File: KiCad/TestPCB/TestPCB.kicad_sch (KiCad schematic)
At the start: 42 parts, among them J1 USB_C_Receptacle_PowerOnly_6P, Q5 2N7000, Q6 2N7000, U1 ESP32-S3-WROOM-1, U1 MCP73831-2-OT, U2 TC1185-xCT

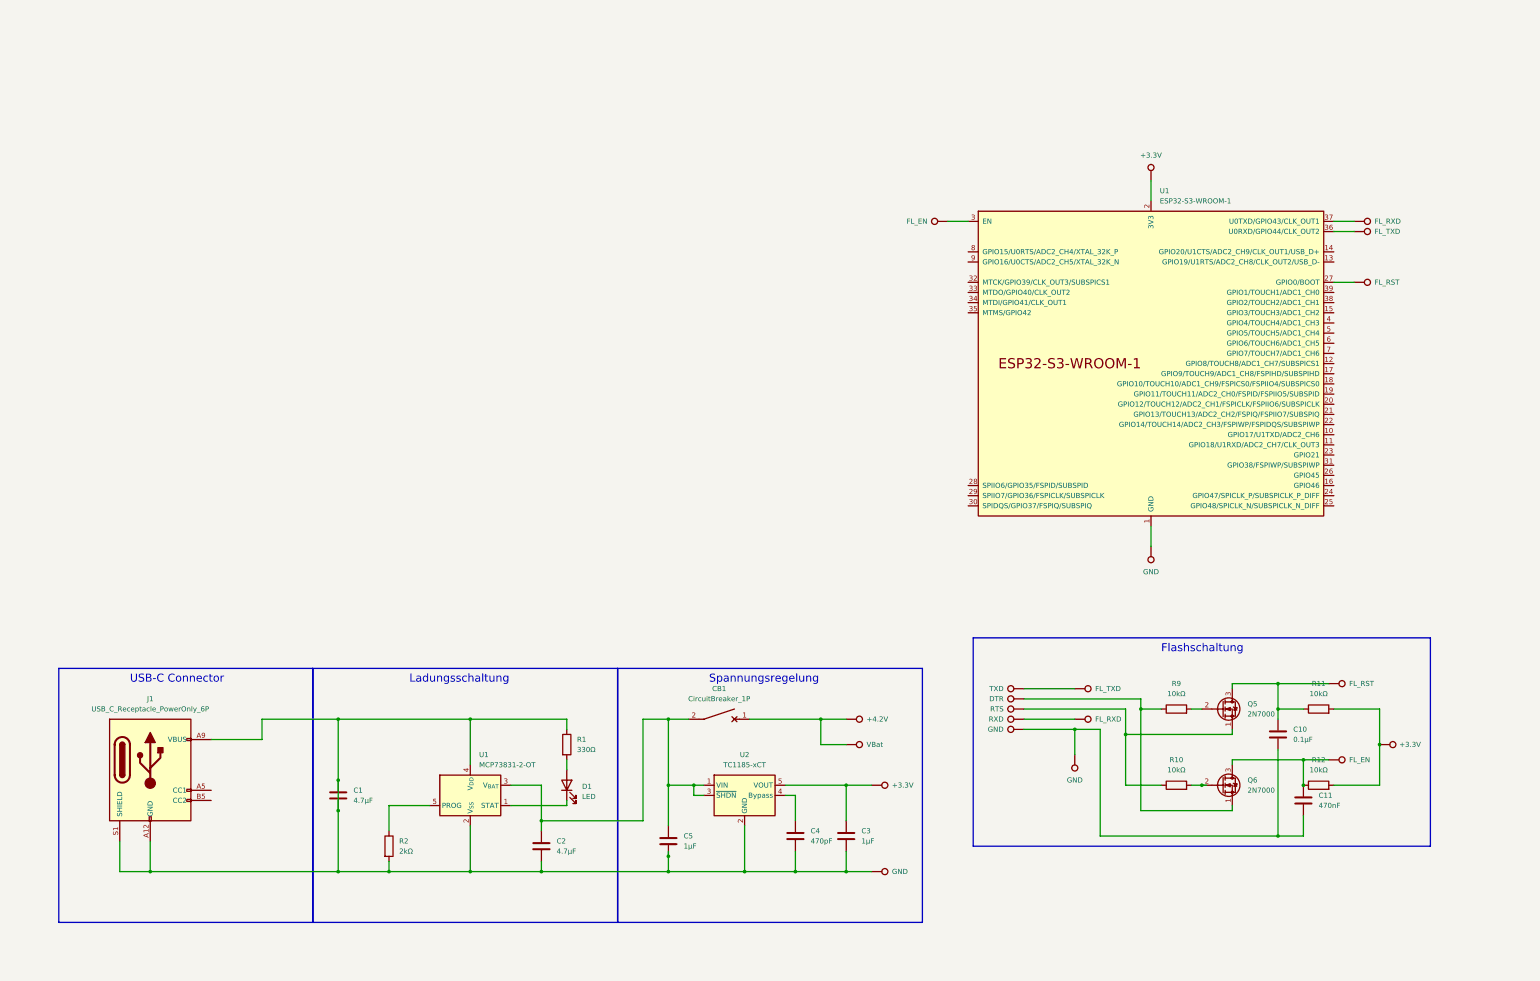
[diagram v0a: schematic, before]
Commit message: ADD: all circuits added
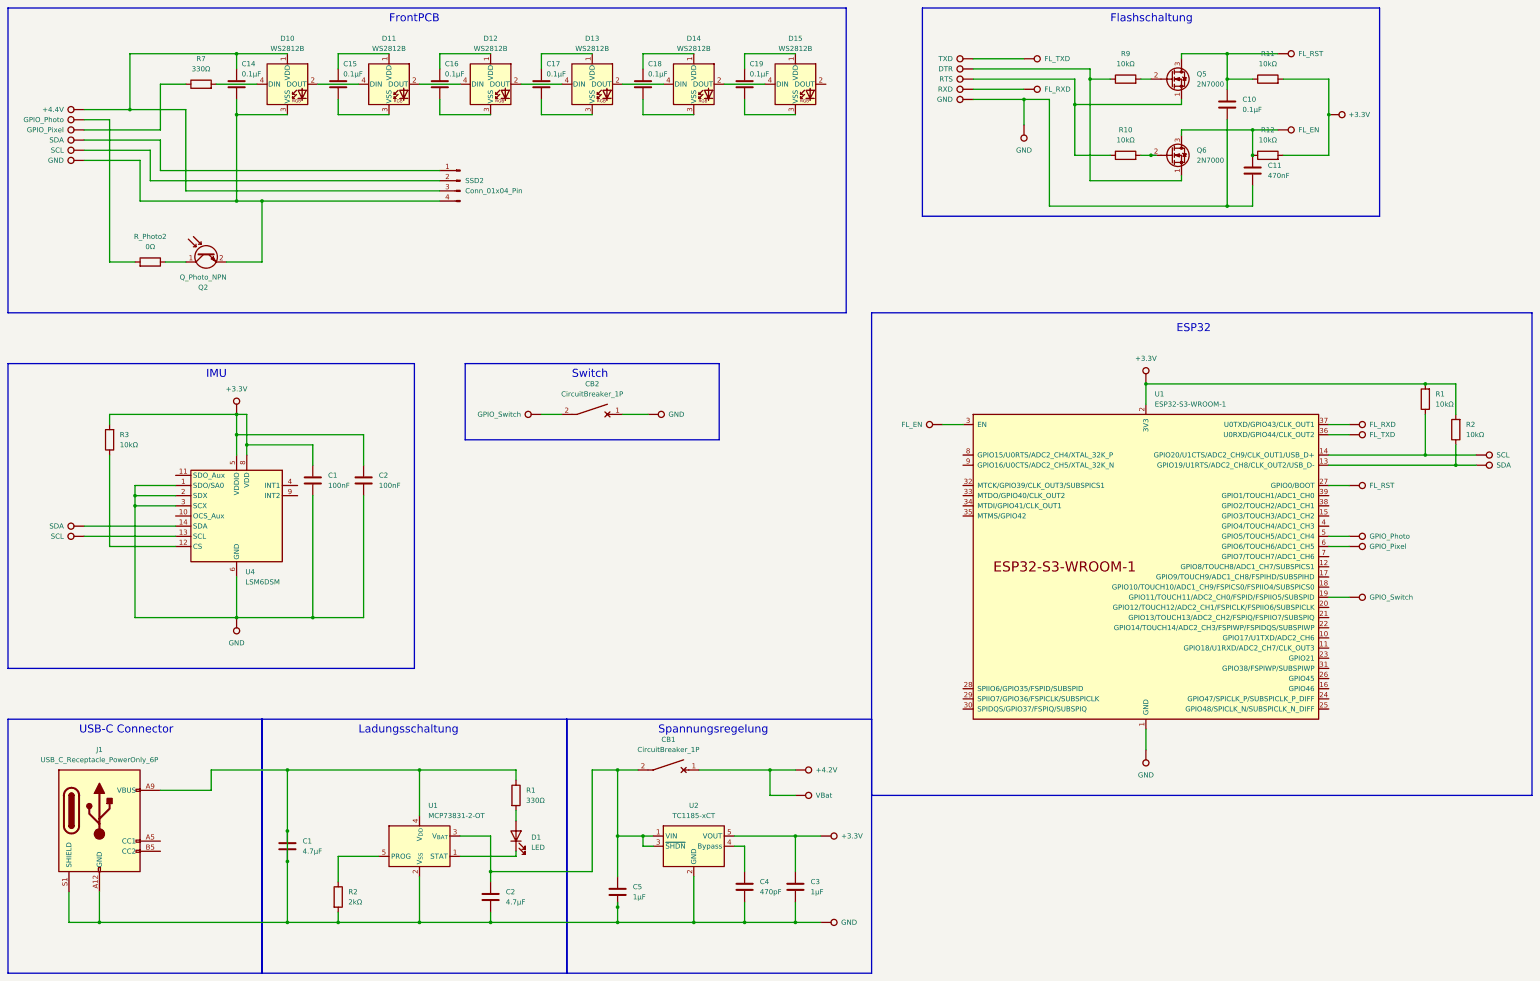
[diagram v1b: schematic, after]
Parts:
- added C1, C2: 100nF, Capacitor_SMD:C_0805_2012Metric, symbol Device:C
- added C14, C15, C16, C17, C18, C19: 0.1µF, Capacitor_SMD:C_0805_2012Metric, symbol Device:C
- added CB2: CircuitBreaker_1P, symbol Device:CircuitBreaker_1P
- added D10, D11, D12, D13, D14, D15: WS2812B, LED_SMD:LED_WS2812B_PLCC4_5.0x5.0mm_P3.2mm, symbol LED:WS2812B
- added Q2: Q_Photo_NPN, LED_SMD:LED_0805_2012Metric, symbol Device:Q_Photo_NPN
- added R1, R2, R3: 10kΩ, Resistor_SMD:R_0805_2012Metric, symbol Device:R
- added R7: 330Ω, Resistor_SMD:R_0805_2012Metric, symbol Device:R
- added R_Photo2: 0Ω, Resistor_SMD:R_0805_2012Metric, symbol Device:R
- added SSD2: Conn_01x04_Pin, Connector_PinHeader_2.54mm:PinHeader_1x04_P2.54mm_Vertical_SMD_Pin1Left, symbol Connector:Conn_01x04_Pin
- added TP22, TP24, TP35: SCL, TestPoint:TestPoint_Pad_2.0x2.0mm, symbol Connector:TestPoint
- added TP23, TP25, TP34: SDA, TestPoint:TestPoint_Pad_2.0x2.0mm, symbol Connector:TestPoint
- added TP26: +3.3V, TestPoint:TestPoint_Pad_2.0x2.0mm, symbol Connector:TestPoint
- added TP27, TP28, TP32: GND, TestPoint:TestPoint_Pad_2.0x2.0mm, symbol Connector:TestPoint
- added TP29, TP30: GPIO_Switch, TestPoint:TestPoint_Pad_2.0x2.0mm, symbol Connector:TestPoint
- added TP31, TP37: GPIO_Photo, TestPoint:TestPoint_Pad_2.0x2.0mm, symbol Connector:TestPoint
- added TP33, TP38: GPIO_Pixel, TestPoint:TestPoint_Pad_2.0x2.0mm, symbol Connector:TestPoint
- added TP36: +4.4V, TestPoint:TestPoint_Pad_2.0x2.0mm, symbol Connector:TestPoint
- added U4: LSM6DSM, Package_LGA:LGA-14_3x2.5mm_P0.5mm_LayoutBorder3x4y, symbol Sensor_Motion:LSM6DSM
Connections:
- net at U1.13 (GPIO19/U1RTS/ADC2_CH8/CLK_OUT2/USB_D-): now also R2.1, TP23.1
- net at U1.14 (GPIO20/U1CTS/ADC2_CH9/CLK_OUT1/USB_D+): now also R1.1, TP22.1
- net at U1.19 (GPIO11/TOUCH11/ADC2_CH0/FSPID/FSPIIO5/SUBSPID): now also TP30.1
- net at TP1.1, U1.2 (3V3): now also R1.2, R2.2
- net at U1.5 (GPIO5/TOUCH5/ADC1_CH4): now also TP37.1
- net at U1.6 (GPIO6/TOUCH6/ADC1_CH5): now also TP38.1
- new net: SSD2.1 (Pin_1), TP34.1
- new net: SSD2.2 (Pin_2), TP35.1
- new net: C14.1, D10.1 (VDD), SSD2.3 (Pin_3), TP36.1
- new net: C14.2, D10.3 (VSS), Q2.2 (E), SSD2.4 (Pin_4), TP32.1
- new net: C16.1, D12.1 (VDD)
- new net: C16.2, D12.3 (VSS)
- new net: CB2.1, TP28.1
- new net: C1.2, C2.2, TP27.1, U4.1 (SDO/SA0), U4.2 (SDX), U4.3 (SCX), U4.6 (GND), U4.7 (GND)
- new net: C18.1, D14.1 (VDD)
- new net: C18.2, D14.3 (VSS)
- new net: R7.1, TP33.1
- new net: D10.4 (DIN), R7.2
- new net: C19.1, D15.1 (VDD)
- new net: C19.2, D15.3 (VSS)
- new net: D14.2 (DOUT), D15.4 (DIN)
- new net: C15.1, D11.1 (VDD)
- new net: C15.2, D11.3 (VSS)
- new net: Q2.1 (C), R_Photo2.1
- new net: R3.1, U4.12 (CS)
- new net: C1.1, C2.1, R3.2, TP26.1, U4.5 (VDDIO), U4.8 (VDD)
- new net: TP24.1, U4.13 (SCL)
- new net: CB2.2, TP29.1
- new net: TP25.1, U4.14 (SDA)
- new net: D10.2 (DOUT), D11.4 (DIN)
- new net: C17.1, D13.1 (VDD)
- new net: D13.2 (DOUT), D14.4 (DIN)
- new net: C17.2, D13.3 (VSS)
- new net: D12.2 (DOUT), D13.4 (DIN)
- new net: R_Photo2.2, TP31.1
- new net: D11.2 (DOUT), D12.4 (DIN)
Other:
- note added: "ESP32"
- note added: "FrontPCB"
- note added: "IMU"
- note added: "Switch"
- moved on the sheet: C1, C10, C11, C2, C3, C4, C5, CB1, D1, J1, Q5, Q6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
